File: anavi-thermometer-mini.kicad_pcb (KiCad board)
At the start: 2 copper layers, 33 x 43.4 mm, 12 parts, among them SW1 SW_DIP_x01, U1 MOUDLE-SEEEDUINO-XIAO-ESP32C6, U2 DS18B20

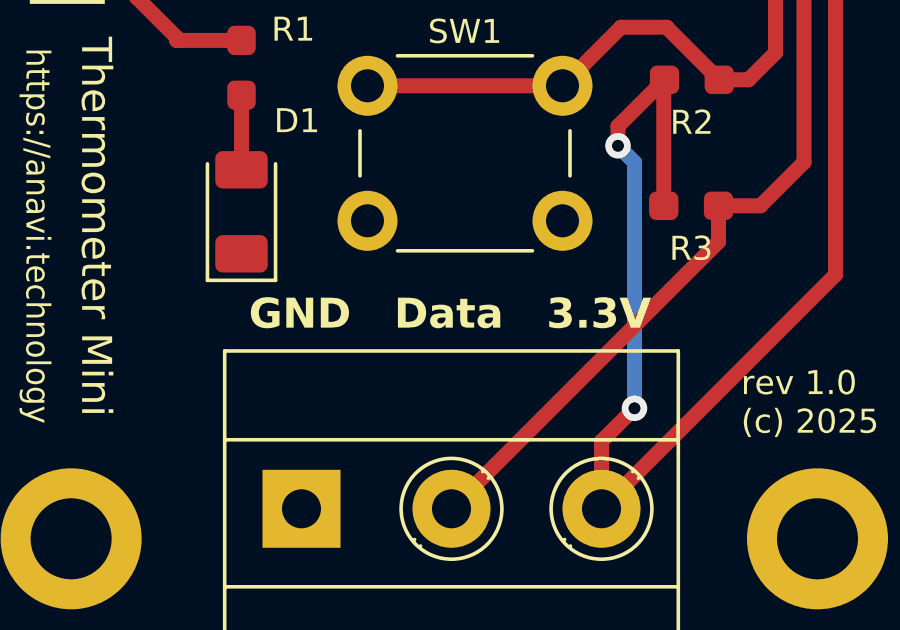
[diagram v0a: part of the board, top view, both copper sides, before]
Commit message: Minor adjustments of the PCB
Signed-off-by: Leon Anavi <leon@anavi.org>
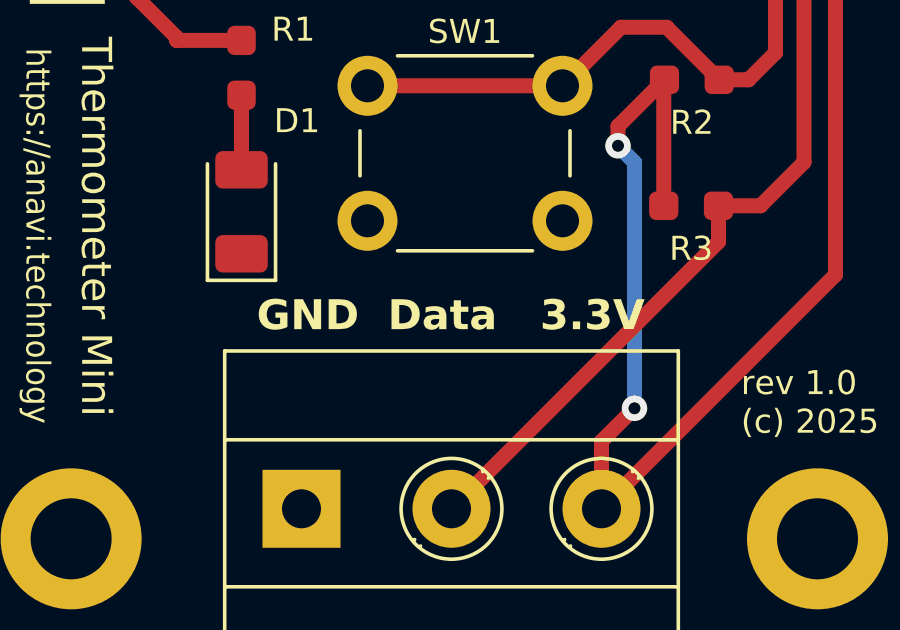
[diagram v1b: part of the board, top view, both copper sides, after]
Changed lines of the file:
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@@
 		)
 	)
-	(gr_text "GND   Data   3.3V"
-		(at 149.35 64.8 0)
+	(gr_text "GND  Data   3.3V"
+		(at 149.375 64.85 0)
 		(layer "F.SilkS")
 		(effects
